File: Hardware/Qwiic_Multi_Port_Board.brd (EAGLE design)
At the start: 25.4 x 25.4 mm, 18 parts, among them J1 QWIIC_RIGHT_ANGLE, J2 QWIIC_RIGHT_ANGLE, J3 QWIIC_RIGHT_ANGLE, J4 QWIIC_RIGHT_ANGLE

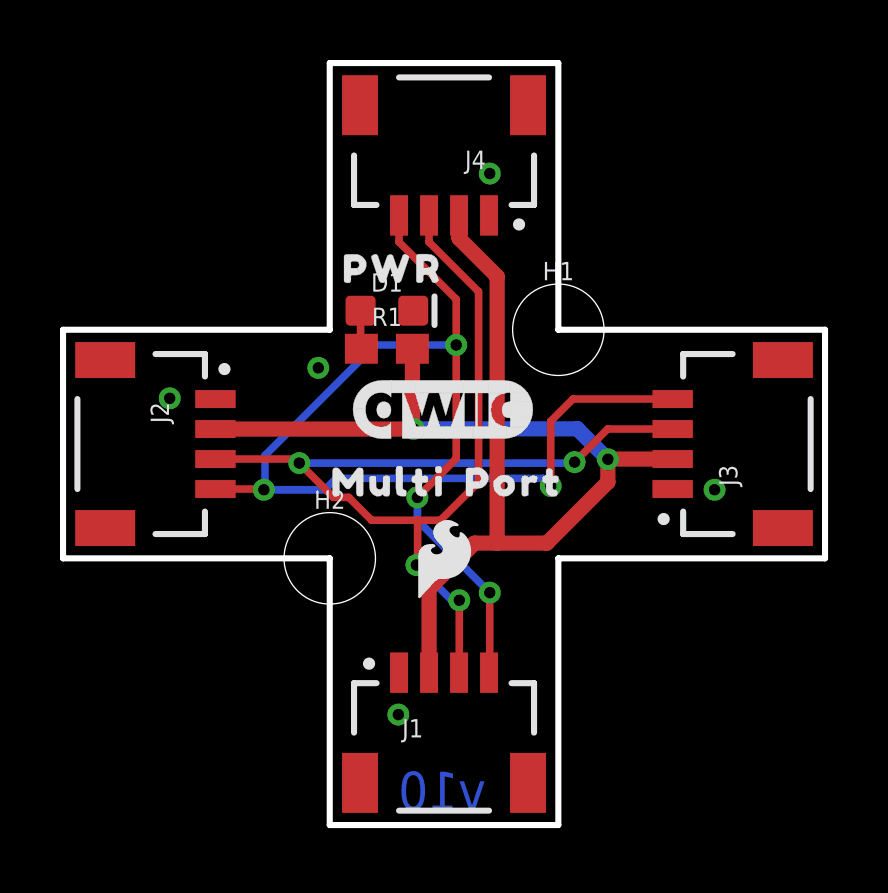
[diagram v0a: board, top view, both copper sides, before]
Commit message: DRC
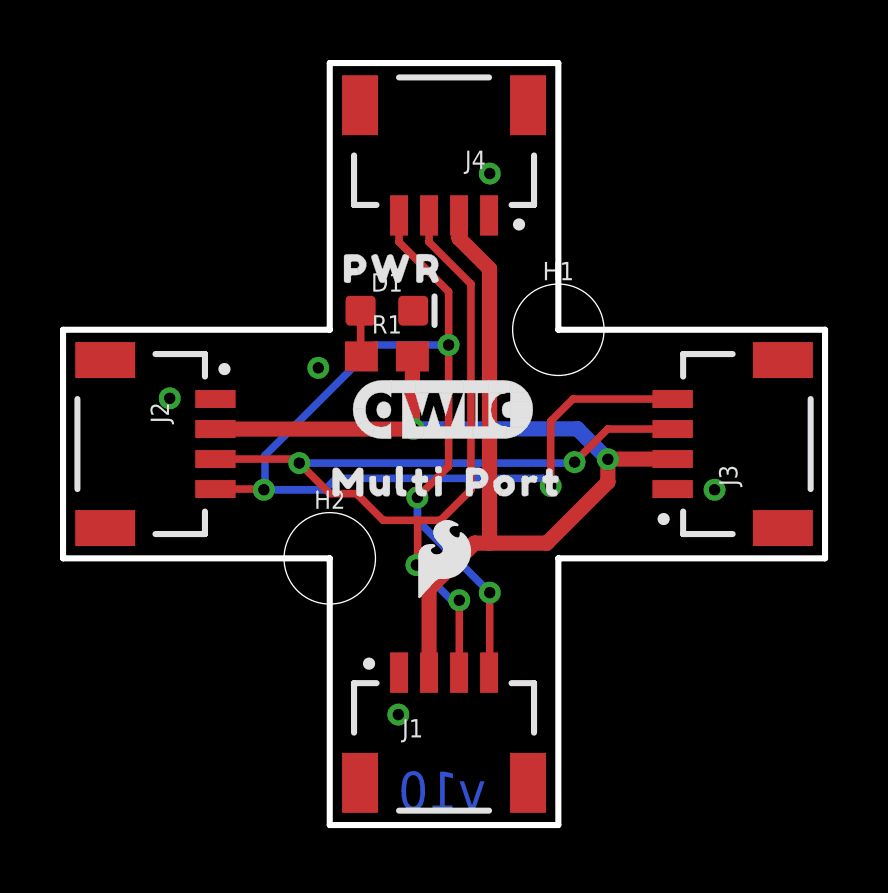
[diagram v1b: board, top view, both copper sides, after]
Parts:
- moved R1 0.25 mm to (10.8, 15.6)
